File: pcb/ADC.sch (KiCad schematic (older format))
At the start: 32 parts, among them J1 Conn_01x02, J2 Screw_Terminal_01x02, J3 Screw_Terminal_01x03, U1 LMH6702MF, U2 ADC080200

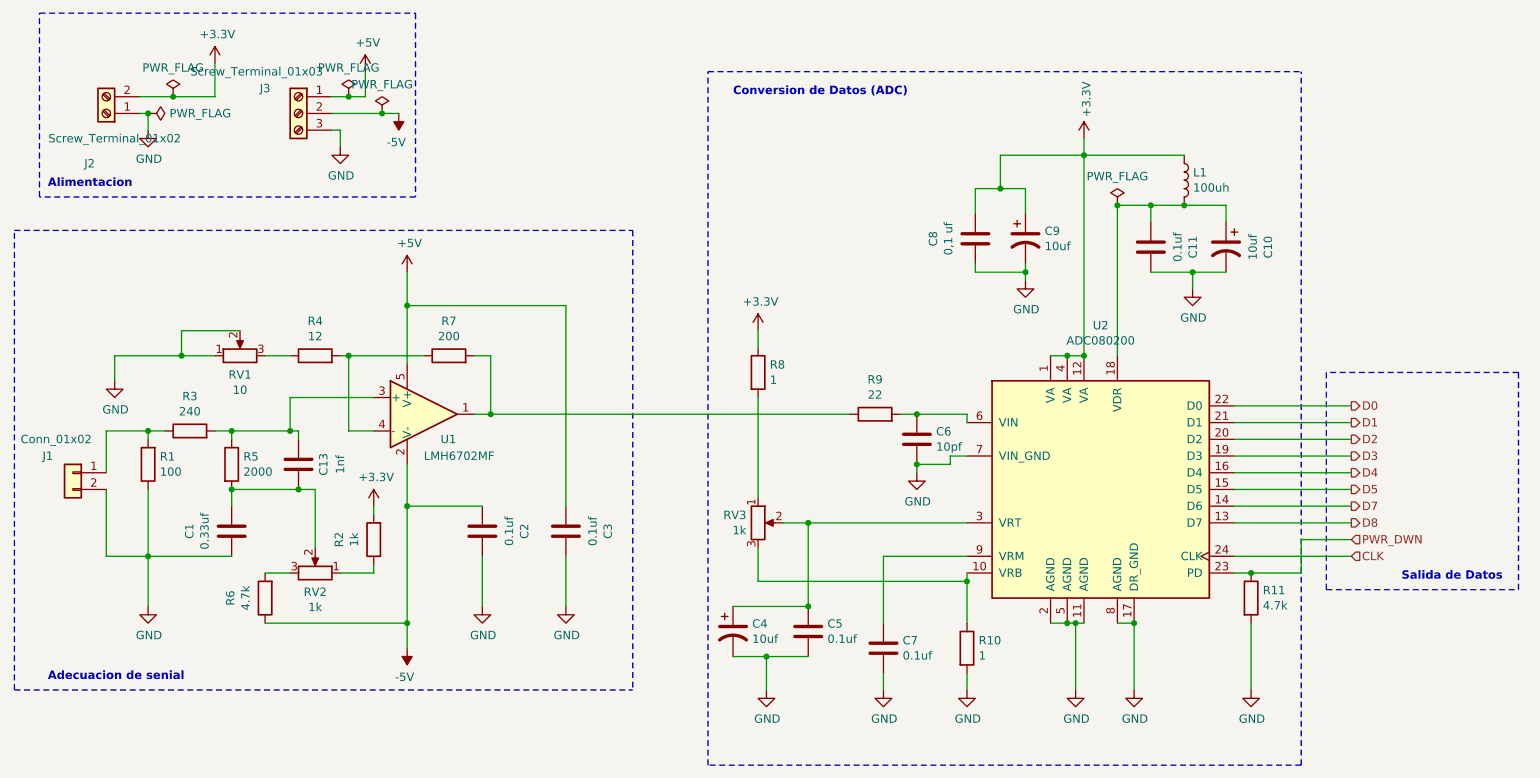
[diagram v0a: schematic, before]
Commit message: correcciones agregadas
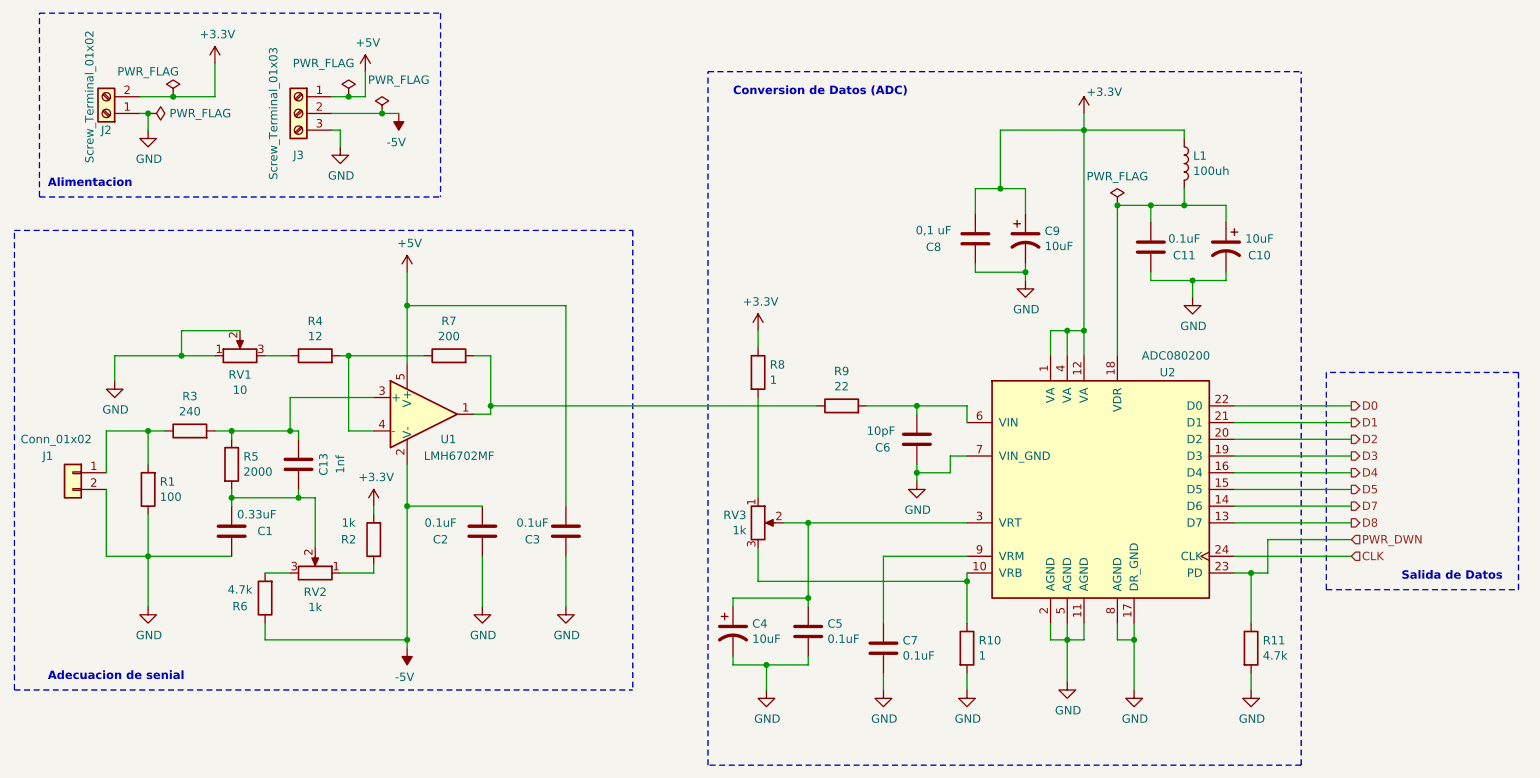
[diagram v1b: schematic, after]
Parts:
- C1: value 0.33uf -> 0.33uF
- C10, C4, C9: value 10uf -> 10uF
- C11, C2, C3, C5, C7: value 0.1uf -> 0.1uF
- C6: value 10pf -> 10pF
- C8: value 0,1 uf -> 0,1 uF
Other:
- moved on the sheet: L1, R1, R11, R9
